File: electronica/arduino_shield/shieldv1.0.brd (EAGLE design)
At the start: 68.6 x 53.3 mm, 35 parts

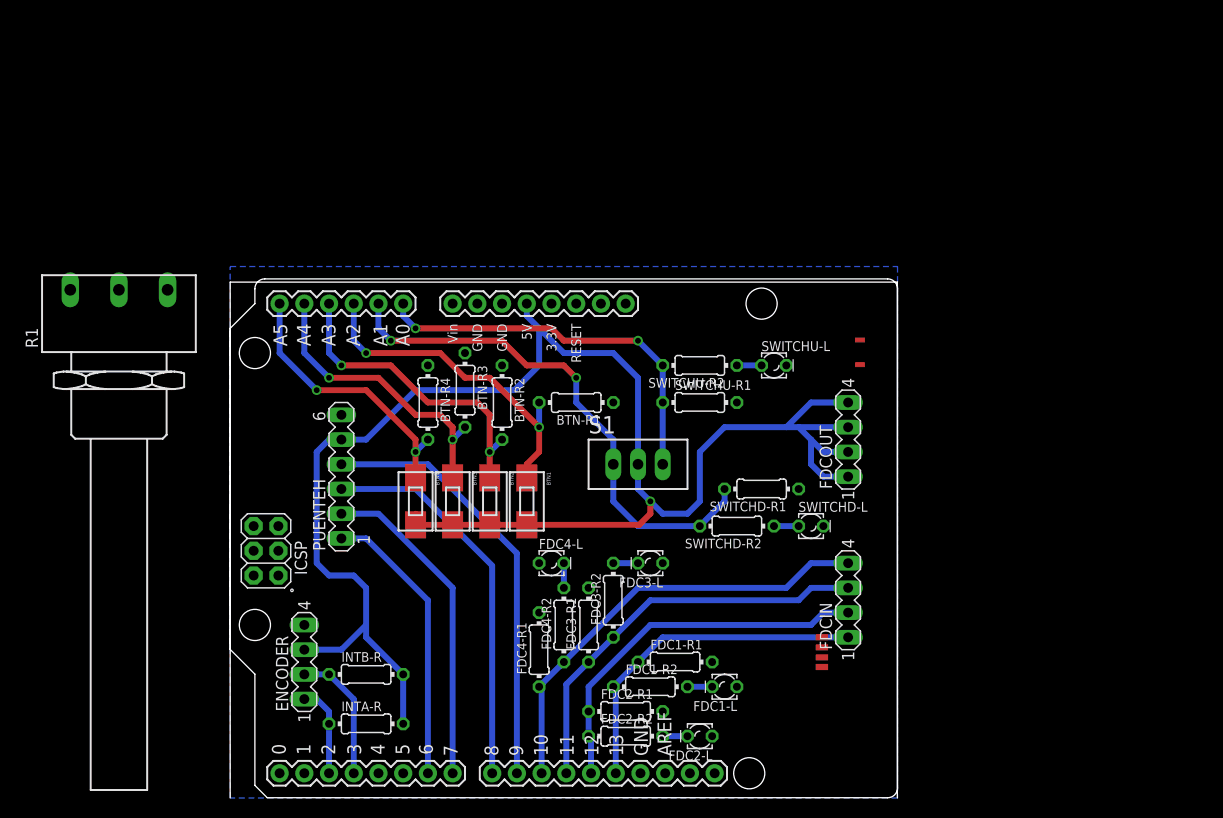
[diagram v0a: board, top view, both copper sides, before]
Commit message: placa
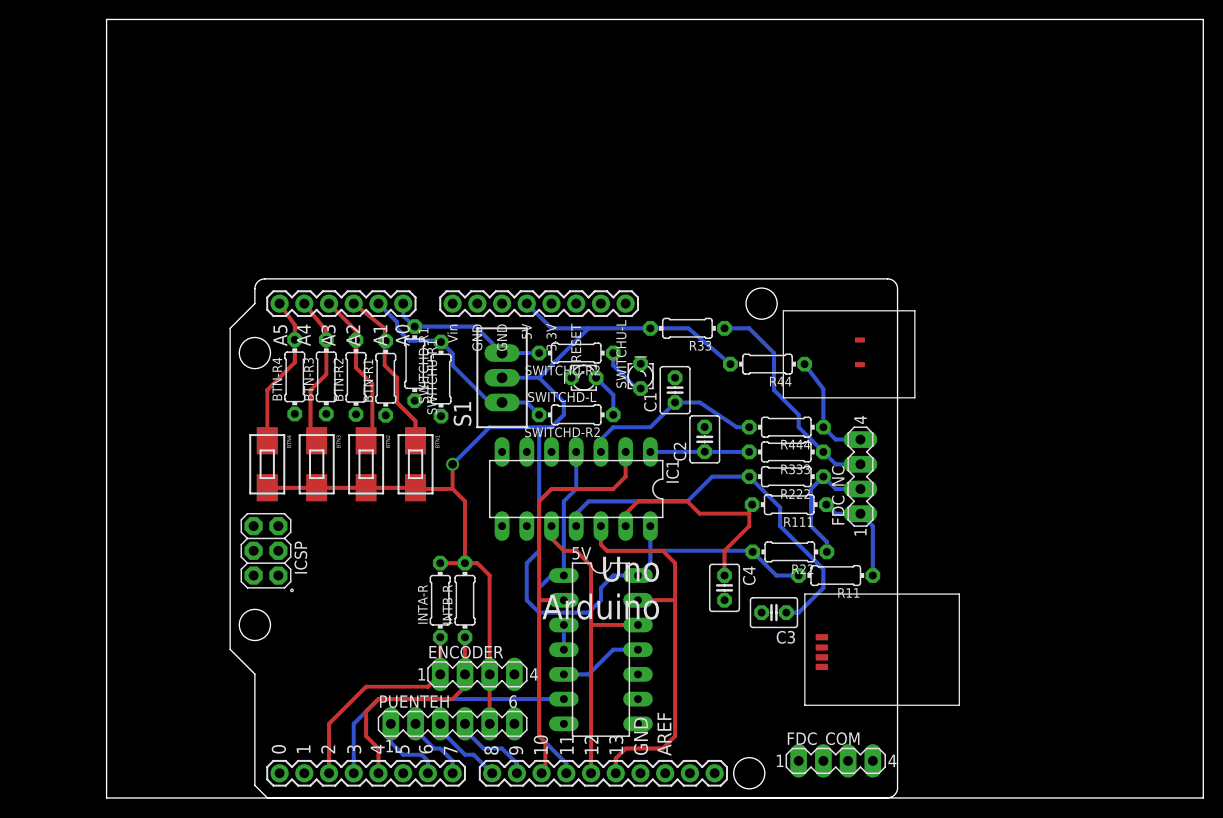
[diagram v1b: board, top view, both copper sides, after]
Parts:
- removed FDC1-L, FDC2-L, FDC3-L, FDC4-L: (no value), eagle-ltspice:LED_LD260
- removed FDC1-R1, FDC1-R2, FDC2-R1, FDC2-R2, FDC3-R1, FDC3-R2, FDC4-R1, FDC4-R2: (no value), resistor:0204/7
- removed FDCIN: 3, con-lstb:MA04-1
- removed FDCOUT: 2, con-lstb:MA04-1
- removed R1: PC16S, piher:PC16S
- added 5V: 7408N, 74ttl-din:DIL14
- added C1, C2, C3, C4: 220n, rcl:C025-030X050
- added FDC_COM: 2, con-lstb:MA04-1
- added FDC_NC: 3, con-lstb:MA04-1
- added IC1: 74HC14N, 74xx-eu:DIL14
- added R11, R111, R22, R222, R33, R333, R44, R444: 5k, rcl:0204/7
- PCB1: device E14_Arduino_revB:ARDUINO_UNO -> uchile_robotics_eagle_library:ARDUINO_UNO
- moved SWITCHD-R1 34.8 mm to (21.7, 43.0), turned to 90 degrees
- moved SWITCHU-R1 29.6 mm to (19.0, 44.6), turned to 270 degrees
- moved SWITCHD-L 27.9 mm to (36.3, 43.2), turned to 180 degrees
- moved PUENTEH 27.9 mm to (22.9, 7.62), turned to 0 degrees
- moved SWITCHD-R2 20.1 mm to (35.6, 39.4)
- moved BTN-R1 19.7 mm to (16.0, 43.1), turned to 90 degrees
- moved ENCODER 17.8 mm to (25.4, 12.7), turned to 0 degrees
- moved S1 16.6 mm to (27.9, 43.2), turned to 90 degrees
- moved BTN4 15.7 mm to (3.81, 34.3)
- moved BTN-R2 15.2 mm to (12.9, 43.2), turned to 90 degrees
- moved INTA-R 14.8 mm to (21.6, 20.3), turned to 90 degrees
- moved BTN3 14.5 mm to (8.89, 34.3)
- moved BTN-R3 14.3 mm to (9.88, 43.3), turned to 90 degrees
- moved BTN-R4 13.9 mm to (6.64, 43.3), turned to 90 degrees
- moved SWITCHU-L 13.7 mm to (42.2, 43.3), turned to 90 degrees
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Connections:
- removed net N$2: FDC2-L.K, FDC2-R2.2
- removed net N$6: FDC3-L.K, FDC3-R2.2
- removed net N$7: FDC4-L.K, FDC4-R2.2
- new net FDC: 5V.6, PCB1.3
- new net N$10: C2.1, IC1.1, R333.2
- new net N$11: FDC_NC.2, R22.1, R222.1
- new net N$12: C3.1, IC1.11, R222.2
- new net N$13: FDC_NC.1, R11.1, R111.1
- new net N$14: C4.1, IC1.13, R111.2
- new net N$19: 5V.11, 5V.5
- new net N$20: 5V.3, 5V.4
- new net N$5: FDC_NC.4, R44.1, R444.1
- new net N$8: C1.1, IC1.3, R444.2
- net 5V: now also 5V.VCC, IC1.14, R11.2, R22.2, R33.2, R44.2; no longer FDCOUT.1, FDCOUT.2, FDCOUT.3, FDCOUT.4
- net FDC1: now also 5V.1, IC1.4, PCB1.11; no longer FDC1-R1.1, FDC1-R2.1, FDCIN.1, PCB1.13
- net FDC2: now also 5V.2, IC1.2, PCB1.10; no longer FDC2-R1.1, FDC2-R2.1, FDCIN.2, PCB1.12
- net FDC3: now also 5V.12, IC1.10, PCB1.12; no longer FDC3-R1.1, FDC3-R2.1, FDCIN.3, PCB1.11
- net FDC4: now also 5V.13, IC1.12, PCB1.13; no longer FDC4-R1.1, FDC4-R2.1, FDCIN.4, PCB1.10
- net GND: now also 5V.GND, C1.2, C2.2, C3.2, C4.2, FDC_COM.1, FDC_COM.2, FDC_COM.3, FDC_COM.4, IC1.7; no longer FDC1-L.A, FDC1-R1.2, FDC2-L.A, FDC2-R1.2, FDC3-L.A, FDC3-R1.2, FDC4-L.A, FDC4-R1.2
- net INTB: now also PCB1.4; no longer PCB1.3
- net N$1: now also FDC_NC.3, R33.1, R333.1; no longer FDC1-L.K, FDC1-R2.2
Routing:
- net N$12: track 0.00 -> 40.1 mm
- net PWM: track 44.4 -> 8.41 mm
- net D1: track 40.1 -> 7.81 mm
- net SWITCHD: track 54.0 -> 22.3 mm, vias 2 -> 0
- net FDC: track 0.00 -> 27.7 mm
- net D2: track 33.6 -> 7.03 mm
- net N$14: track 0.00 -> 23.5 mm
- net SWITCHU: track 40.2 -> 16.8 mm, vias 2 -> 0
- net D3: track 29.3 -> 7.77 mm
- net N$1: track 2.54 -> 22.7 mm
- net N$8: track 0.00 -> 18.9 mm
- net BTN-IN1: track 34.8 -> 17.1 mm, vias 2 -> 0
- net 5V: track 174.4 -> 157.8 mm
- net BTN-IN2: track 32.5 -> 16.2 mm, vias 2 -> 0
- net BTN-IN3: track 30.5 -> 15.8 mm, vias 2 -> 0
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- removed copper zone on layer 16, net GND
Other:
- board size 68.6 x 53.3 mm -> 112.7 x 80 mm
